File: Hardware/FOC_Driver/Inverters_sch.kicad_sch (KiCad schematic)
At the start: 6 parts, among them Q4 CSD18540Q5B, Q5 CSD18540Q5B, Q6 CSD18540Q5B, Q7 CSD18540Q5B, Q8 CSD18540Q5B, Q9 CSD18540Q5B

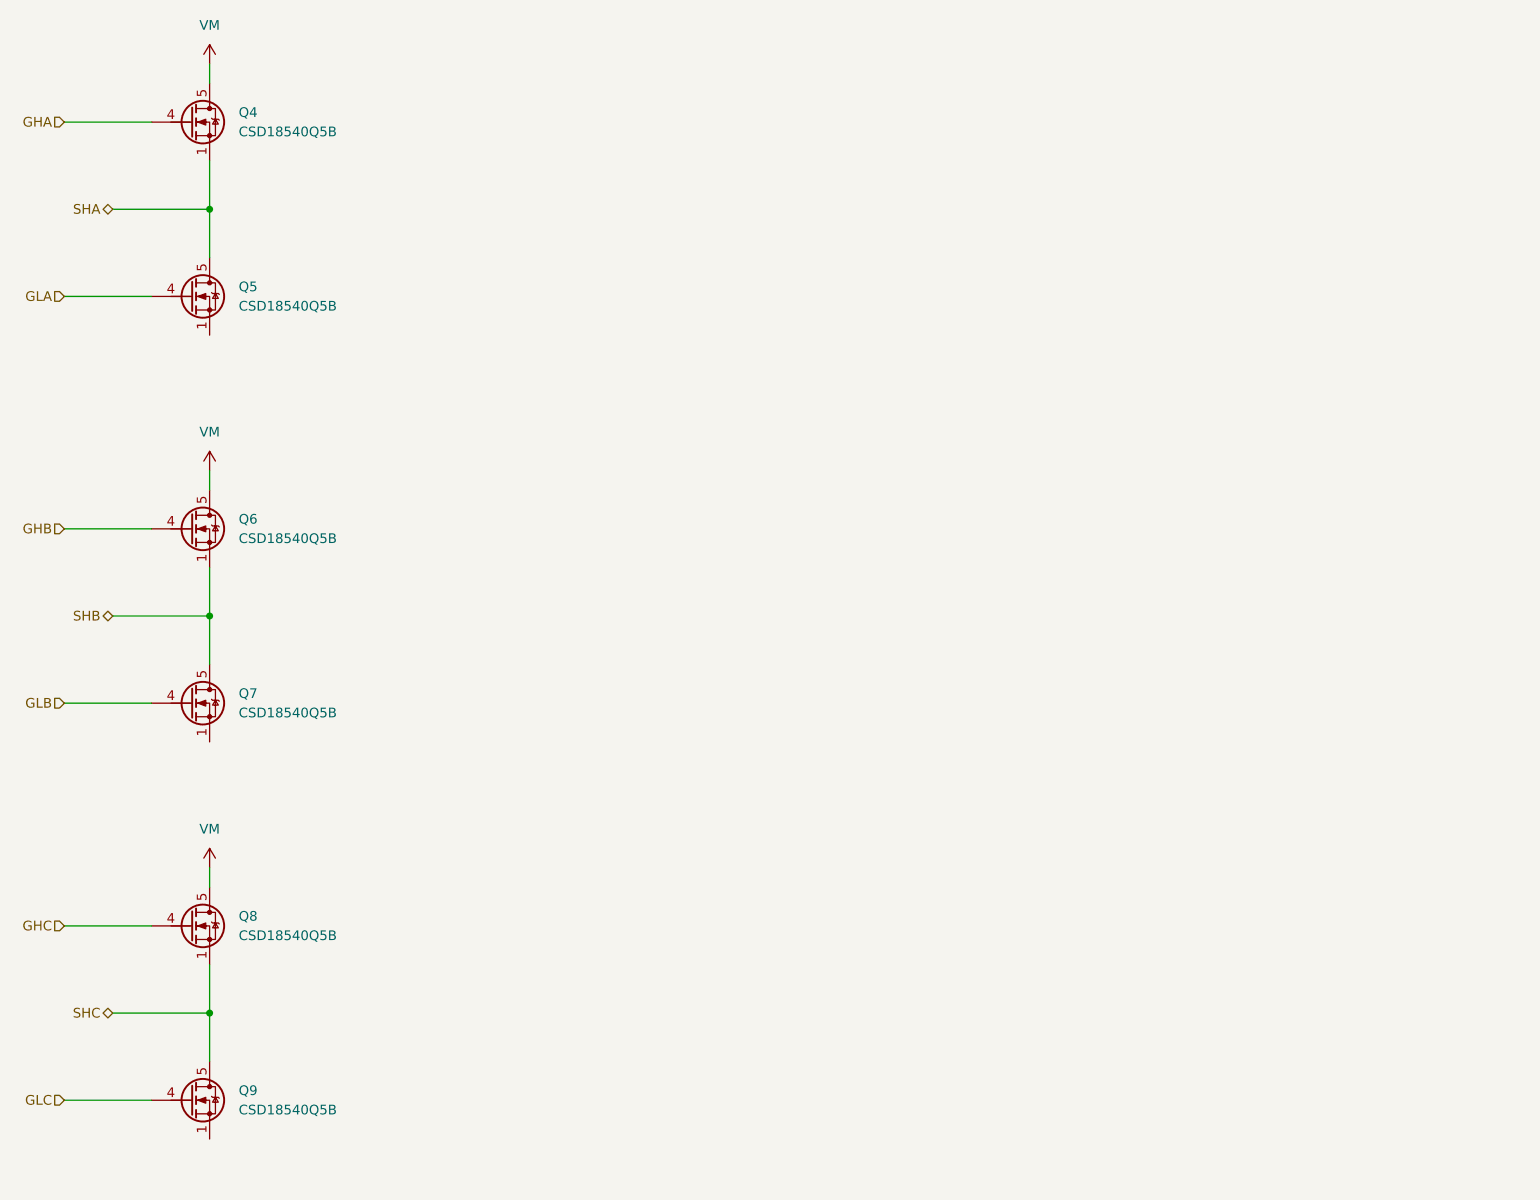
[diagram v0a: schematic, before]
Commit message: schematic updates
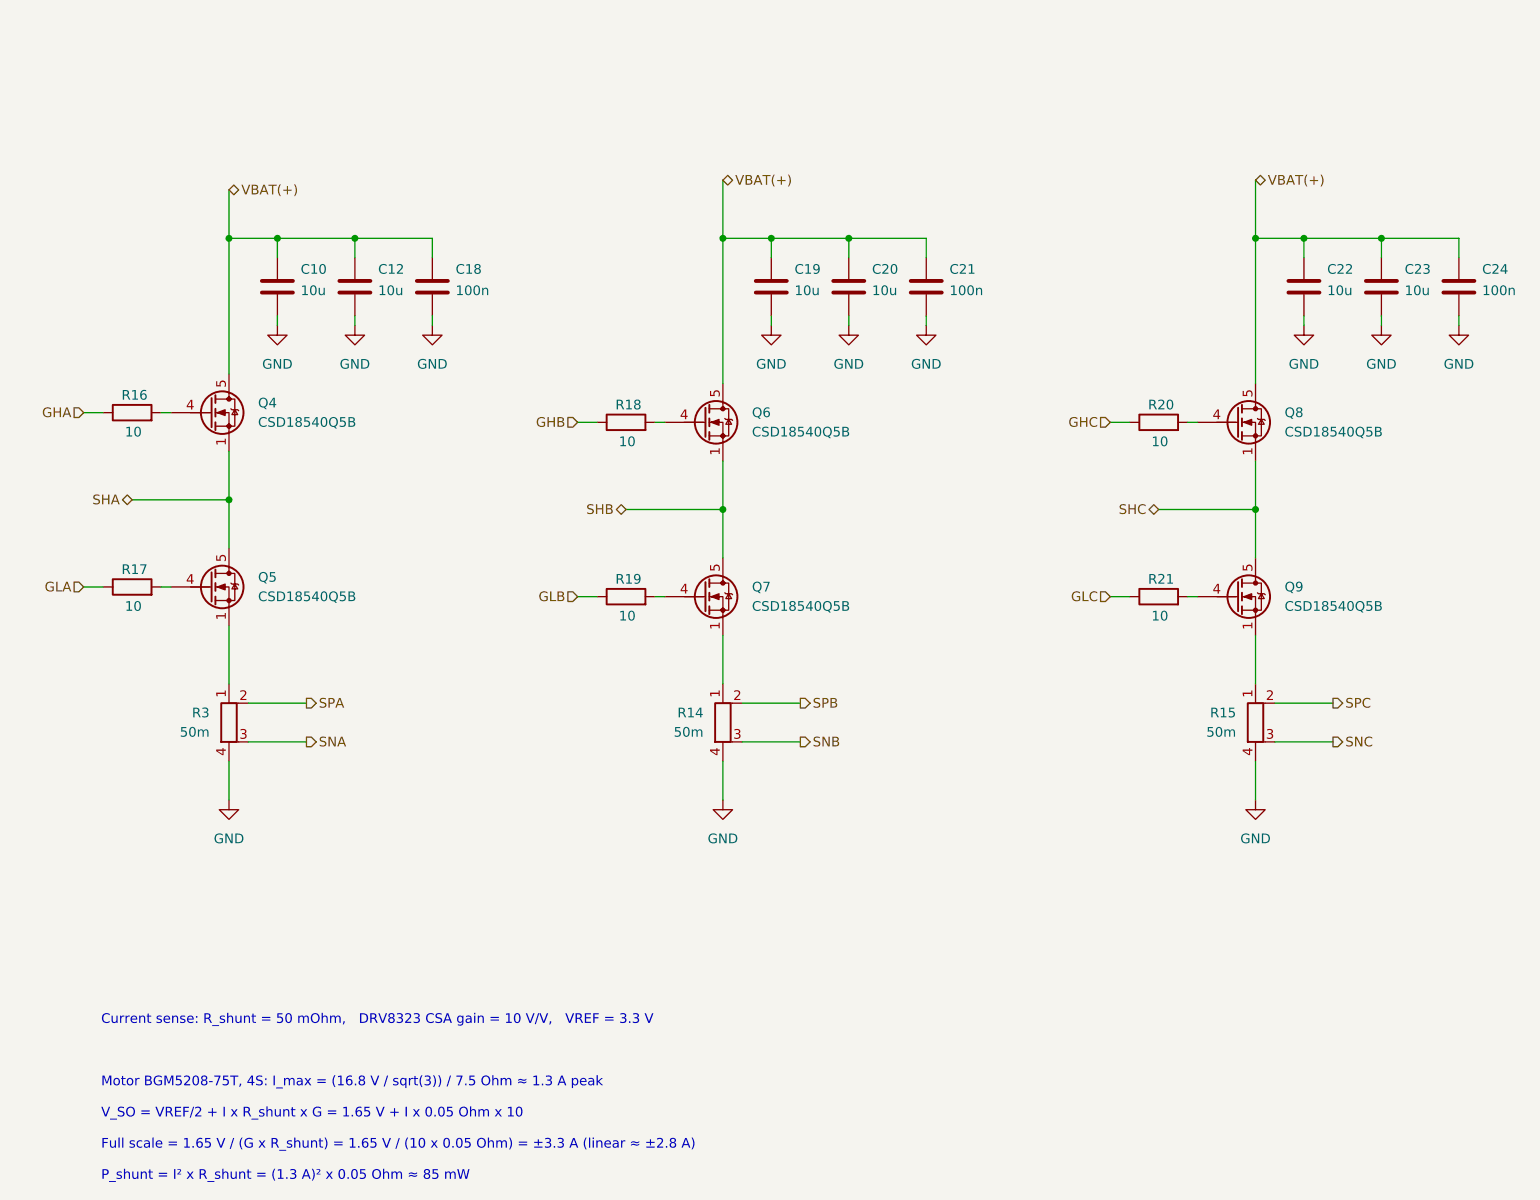
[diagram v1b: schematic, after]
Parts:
- added C10, C12, C19, C20, C22, C23: 10u, Capacitor_SMD:C_1206_3216Metric, symbol Device:C
- added C18, C21, C24: 100n, Capacitor_SMD:C_0603_1608Metric, symbol Device:C
- added R14, R15, R3: 50m, Resistor_SMD:R_Shunt_Vishay_WSK2512_6332Metric_T1.19mm, symbol Device:R_Shunt
- added R16, R17, R18, R19, R20, R21: 10, eResistor:R_0603_1608Metric, symbol Device:R
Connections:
- net GHA: now also R16.1; no longer Q4.4 (G)
- net GHB: now also R18.1; no longer Q6.4 (G)
- net GHC: now also R20.1; no longer Q8.4 (G)
- net GLA: now also R17.1; no longer Q5.4 (G)
- net GLB: now also R19.1; no longer Q7.4 (G)
- net GLC: now also R21.1; no longer Q9.4 (G)
- net at Q9.1 (S), Q9.2 (S), Q9.3 (S): now also R15.1
- net at Q5.1 (S), Q5.2 (S), Q5.3 (S): now also R3.1
- net at Q7.1 (S), Q7.2 (S), Q7.3 (S): now also R14.1
- net VM renamed VBAT(+)
- net VBAT(+): now also C10.1, C12.1, C18.1, C19.1, C20.1, C21.1, C22.1, C23.1, C24.1
- new net: Q6.4 (G), R18.2
- new net: Q9.4 (G), R21.2
- new net: Q5.4 (G), R17.2
- new net: Q4.4 (G), R16.2
- new net: Q8.4 (G), R20.2
- new net: Q7.4 (G), R19.2
- new net GND: C10.2, C12.2, C18.2, C19.2, C20.2, C21.2, C22.2, C23.2, C24.2, R14.4, R15.4, R3.4
- new net SNA: R3.3
- new net SNB: R14.3
- new net SNC: R15.3
- new net SPA: R3.2
- new net SPB: R14.2
- new net SPC: R15.2
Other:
- note added: "Current sense: R_shunt = 50 mOhm, DRV8323 CSA gain = 10 V/V, VREF = 3.3 V Motor BGM5208-75T, 4S: I_max = (16.8 V / sqrt(3)) / 7.5 Ohm ≈ 1.3 A peak V_SO = VREF/2 + I x R_shunt x G = 1.65 V + I x 0.05 Ohm x 10 Full scale = 1.65 V / (G x R_shunt) = 1.65 V / (10 x 0.05 Ohm) = ±3.3 A (linear ≈ ±2.8 A) P_shunt = I² x R_shunt = (1.3 A)² x 0.05 Ohm ≈ 85 mW"
- moved on the sheet: Q4, Q5, Q6, Q7, Q8, Q9
